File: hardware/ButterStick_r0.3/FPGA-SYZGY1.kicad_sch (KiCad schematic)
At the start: 1 part, among them U4 ECP5UM5G_85_CABGA381

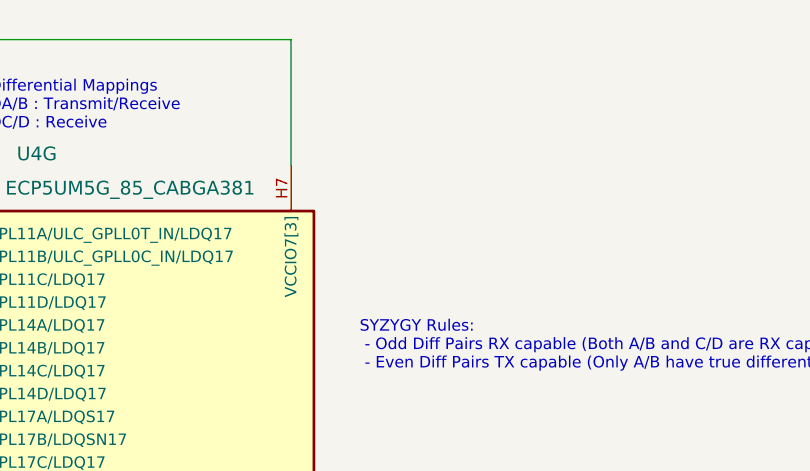
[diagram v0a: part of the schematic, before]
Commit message: hw.r0d3: complete first pass of routing
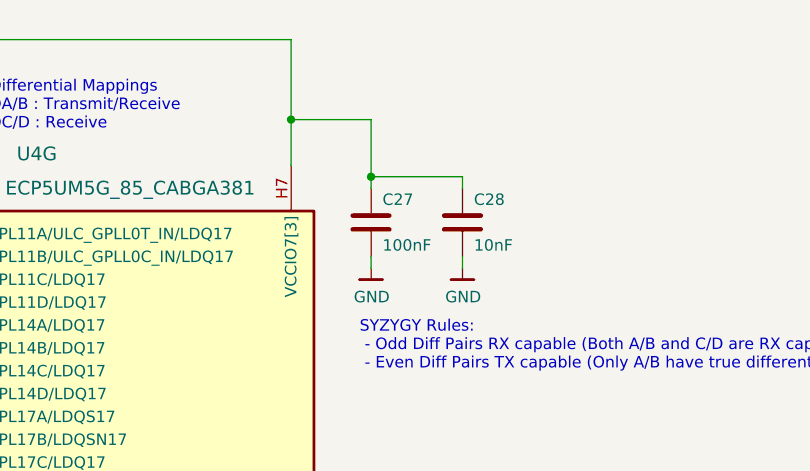
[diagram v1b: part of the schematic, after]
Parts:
- added C27: 100nF, Capacitor_SMD:C_0402_1005Metric, symbol Device:C
- added C28: 10nF, Capacitor_SMD:C_0402_1005Metric, symbol Device:C
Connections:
- net VIO1: now also C27.1, C28.1
- new net GND: C27.2, C28.2
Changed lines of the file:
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@@
-(kicad_sch (version 20200608) (host eeschema "5.99.0-unknown-08c61e6~101~ubuntu18.04.1")
-  (page 1 19)
+(kicad_sch (version 20200618) (host eeschema "5.99.0-unknown-476558e~101~ubuntu18.04.1")
+  (page 10 19)
   (paper "A4")
-  (bus_entry (at 104.14 52.07) (size 2.54 -2.54))
+  (junction (at 157.48 58.42) (diameter 0) (color 0 0 0 0))
+  (junction (at 166.37 64.77) (diameter 0) (color 0 0 0 0))
+  (bus_entry (at 104.14 52.07) (size 2.54 -2.54)
+    (stroke (width 0.1524) (type solid) (color 0 0 0 0))
+  )
   (wire (pts (xy 105.41 71.12) (xy 119.38 71.12))
     (stroke (width 0) (type solid) (color 0 0 0 0))
@@
     (stroke (width 0) (type solid) (color 0 0 0 0))
   )
-  (wire (pts (xy 157.48 49.53) (xy 157.48 63.5))
+  (wire (pts (xy 157.48 49.53) (xy 157.48 58.42))
+    (stroke (width 0) (type solid) (color 0 0 0 0))
+  )
+  (wire (pts (xy 157.48 58.42) (xy 157.48 63.5))
+    (stroke (width 0) (type solid) (color 0 0 0 0))
+  )
+  (wire (pts (xy 157.48 58.42) (xy 166.37 58.42))
+    (stroke (width 0) (type solid) (color 0 0 0 0))
+  )
+  (wire (pts (xy 166.37 58.42) (xy 166.37 64.77))
+    (stroke (width 0) (type solid) (color 0 0 0 0))
+  )
+  (wire (pts (xy 166.37 64.77) (xy 166.37 66.04))
+    (stroke (width 0) (type solid) (color 0 0 0 0))
+  )
+  (wire (pts (xy 166.37 64.77) (xy 176.53 64.77))
+    (stroke (width 0) (type solid) (color 0 0 0 0))
+  )
+  (wire (pts (xy 166.37 73.66) (xy 166.37 74.93))
+    (stroke (width 0) (type solid) (color 0 0 0 0))
+  )
+  (wire (pts (xy 176.53 66.04) (xy 176.53 64.77))
+    (stroke (width 0) (type solid) (color 0 0 0 0))
+  )
+  (wire (pts (xy 176.53 74.93) (xy 176.53 73.66))
     (stroke (width 0) (type solid) (color 0 0 0 0))
   )
@@
     (effects (font (size 1.27 1.27)) (justify right))
   )
+  (symbol (lib_id "gkl_power:GND") (at 166.37 74.93 0) (unit 1)
+    (in_bom yes) (on_board yes)
+    (property "Reference" "#PWR0213" (id 0) (at 166.37 81.28 0)
+      (effects (font (size 1.27 1.27)) hide)
+    )
+    (property "Value" "GND" (id 1) (at 166.4462 78.1304 0))
+    (property "Footprint" "" (id 2) (at 163.83 83.82 0)
+      (effects (font (size 1.27 1.27)) hide)
+    )
+    (property "Datasheet" "" (id 3) (at 166.37 74.93 0)
+      (effects (font (size 1.27 1.27)) hide)
+    )
+  )
+  (symbol (lib_id "gkl_power:GND") (at 176.53 74.93 0) (unit 1)
+    (in_bom yes) (on_board yes)
+    (property "Reference" "#PWR0212" (id 0) (at 176.53 81.28 0)
+      (effects (font (size 1.27 1.27)) hide)
+    )
+    (property "Value" "GND" (id 1) (at 176.6062 78.1304 0))
+    (property "Footprint" "" (id 2) (at 173.99 83.82 0)
+      (effects (font (size 1.27 1.27)) hide)
+    )
+    (property "Datasheet" "" (id 3) (at 176.53 74.93 0)
+      (effects (font (size 1.27 1.27)) hide)
+    )
+  )
+  (symbol (lib_id "Device:C") (at 166.37 69.85 0) (unit 1)
+    (in_bom yes) (on_board yes)
+    (property "Reference" "C27" (id 0) (at 167.64 67.31 0)
+      (effects (font (size 1.27 1.27)) (justify left))
+    )
+    (property "Value" "100nF" (id 1) (at 167.64 72.39 0)
+      (effects (font (size 1.27 1.27)) (justify left))
+    )
+    (property "Footprint" "Capacitor_SMD:C_0402_1005Metric" (id 2) (at 167.3352 73.66 0)
+      (effects (font (size 1.27 1.27)) hide)
+    )
+    (property "Datasheet" "" (id 3) (at 166.37 69.85 0)
+      (effects (font (size 1.27 1.27)) hide)
+    )
+    (property "SN-DK" "1276-1002-1-ND" (id 4) (at 16.51 246.38 0)
+      (effects (font (size 1.27 1.27)) hide)
+    )
+    (property "PN" "CL05B104KP5NNNC" (id 5) (at 16.51 246.38 0)
+      (effects (font (size 1.27 1.27)) hide)
+    )
+    (property "Mfg" "Samsung Electro-Mechanics" (id 6) (at 19.05 245.11 0)
+      (effects (font (size 1.27 1.27)) hide)
+    )
+  )
+  (symbol (lib_id "Device:C") (at 176.53 69.85 0) (unit 1)
+    (in_bom yes) (on_board yes)
+    (property "Reference" "C28" (id 0) (at 177.8 67.31 0)
+      (effects (font (size 1.27 1.27)) (justify left))
+    )
+    (property "Value" "10nF" (id 1) (at 177.8 72.39 0)
+      (effects (font (size 1.27 1.27)) (justify left))
+    )
+    (property "Footprint" "Capacitor_SMD:C_0402_1005Metric" (id 2) (at 177.4952 73.66 0)
+      (effects (font (size 1.27 1.27)) hide)
+    )
+    (property "Datasheet" "" (id 3) (at 176.53 69.85 0)
+      (effects (font (size 1.27 1.27)) hide)
+    )
+    (property "SN-DK" "1276-1002-1-ND" (id 4) (at 26.67 246.38 0)
+      (effects (font (size 1.27 1.27)) hide)
+    )
+    (property "PN" "CL05B103KP5NNNC" (id 5) (at 26.67 246.38 0)
+      (effects (font (size 1.27 1.27)) hide)
+    )
+    (property "Mfg" "Samsung Electro-Mechanics" (id 6) (at 19.05 245.11 0)
+      (effects (font (size 1.27 1.27)) hide)
+    )
+  )
   (symbol (lib_id "gkl_lattice:ECP5UM5G_85_CABGA381") (at 119.38 71.12 0) (unit 7)
